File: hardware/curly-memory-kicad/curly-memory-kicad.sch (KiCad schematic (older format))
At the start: 18 parts

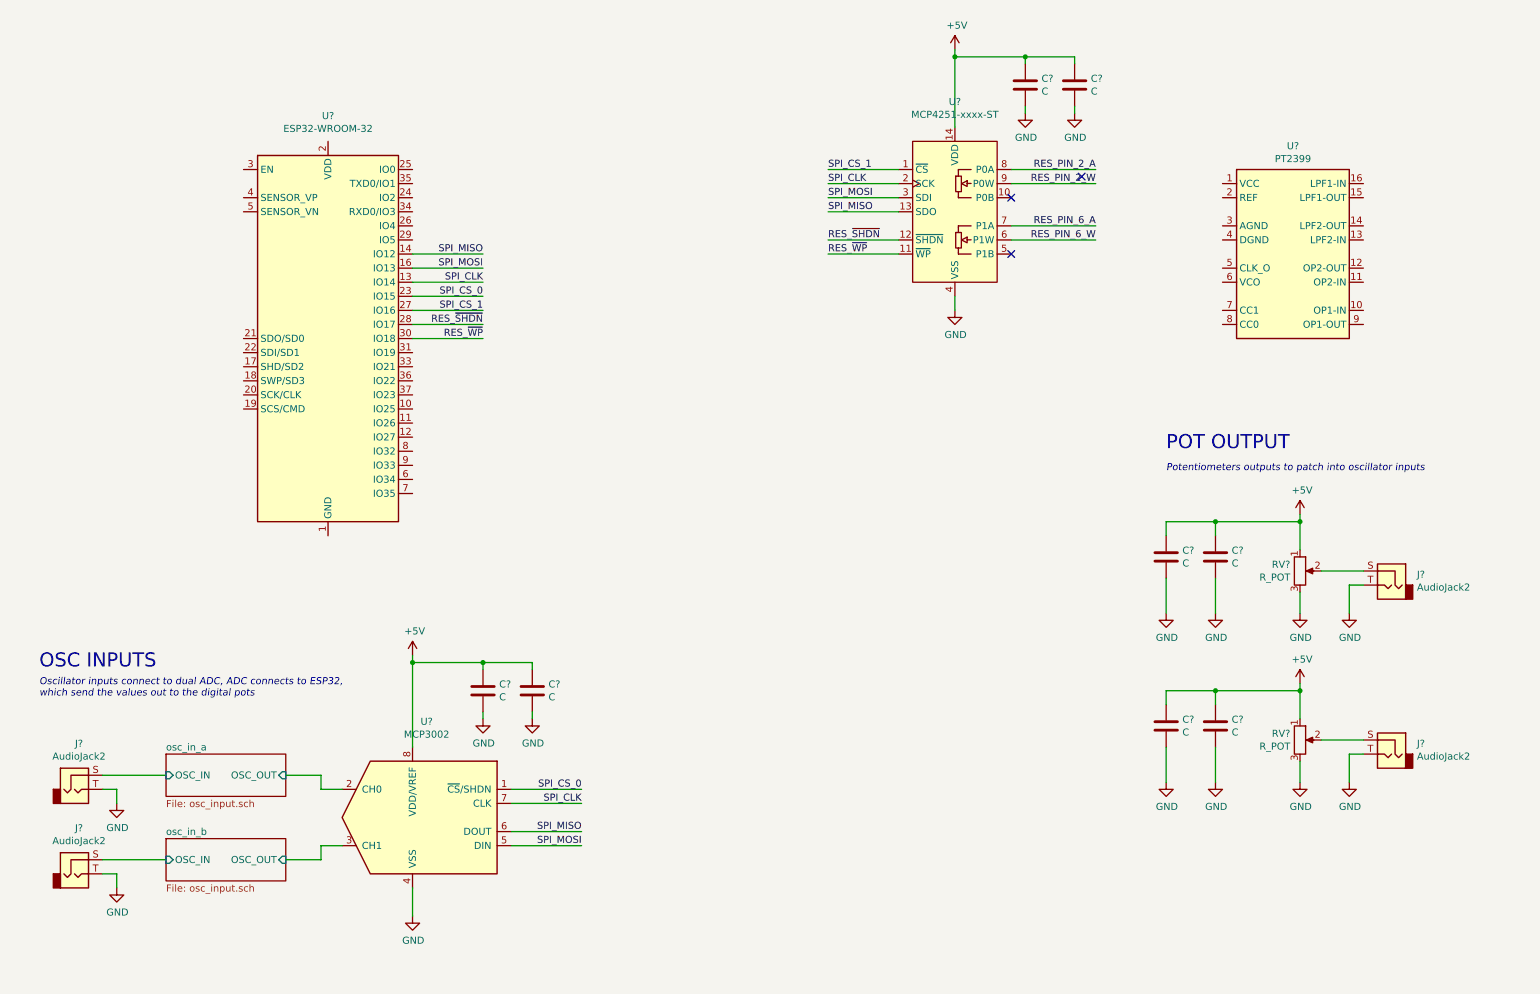
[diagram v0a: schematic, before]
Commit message: hardware update to relfect latest version of projectm gitignore updated to ignore *-bak files
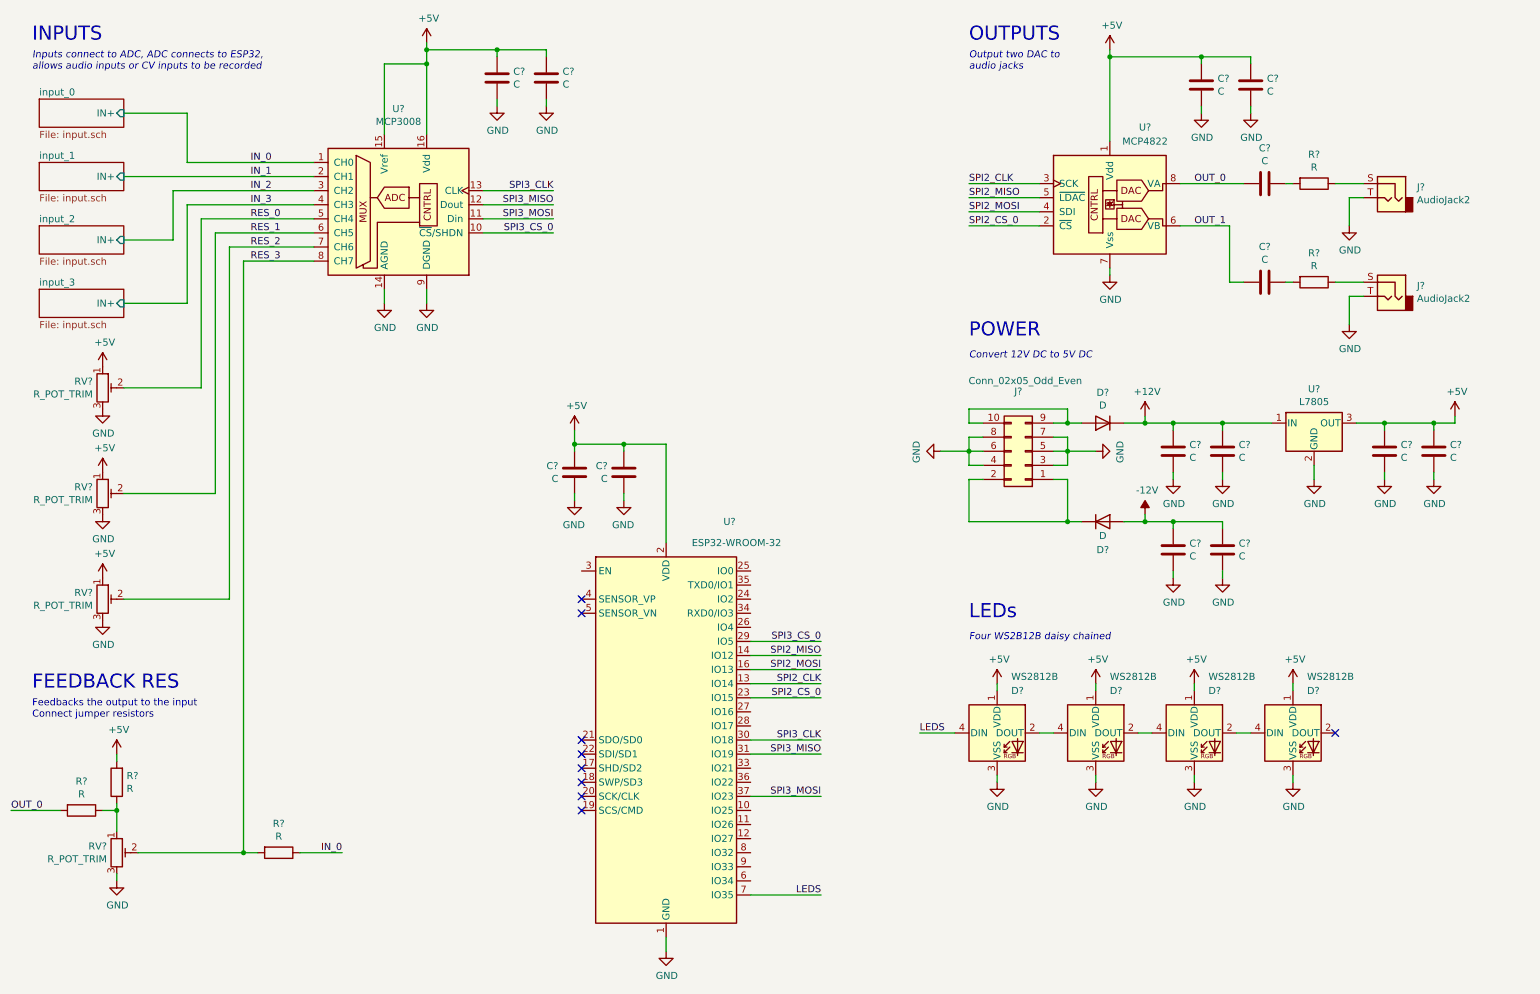
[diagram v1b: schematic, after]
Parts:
- removed C? (x6): C, symbol Device:C
- removed J? (x2): AudioJack2, symbol Connector:AudioJack2
- removed RV? (x2): R_POT, symbol Device:R_POT
- removed U?: MCP3002, symbol Analog_ADC:MCP3002
- removed U?: MCP4251-xxxx-ST, Package_SO:TSSOP-14_4.4x5mm_P0.65mm, symbol Potentiometer_Digital:MCP4251-xxxx-ST
- removed U?: PT2399, symbol Audio:PT2399
- added C? (x12): C, symbol Device:C
- added D? (x4): WS2812B, LED_SMD:LED_WS2812B_PLCC4_5.0x5.0mm_P3.2mm, symbol LED:WS2812B
- added D? (x2): D, symbol Device:D
- added J?: Conn_02x05_Odd_Even, symbol Connector_Generic:Conn_02x05_Odd_Even
- added R? (x5): R, symbol Device:R
- added RV? (x4): R_POT_TRIM, symbol Device:R_POT_TRIM
- added U?: MCP3008, symbol Analog_ADC:MCP3008
- added U?: MCP4822, symbol Analog_DAC:MCP4822
- added U?: L7805, symbol Regulator_Linear:L7805
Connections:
- net +5V: now also U?.2 (VDD), C?.1, C?.1, C?.1, C?.1, C?.1, C?.1, D?.1 (VDD), D?.1 (VDD), D?.1 (VDD), D?.1 (VDD), R?.2, RV?.1, RV?.1, RV?.1, U?.1 (Vdd), U?.15 (Vref), U?.16 (Vdd), U?.3 (OUT)
- net GND: now also U?.1 (GND), U?.15 (GND), U?.38 (GND), U?.39 (GND), C?.2, C?.2, C?.2, C?.2, C?.2, C?.2, C?.2, C?.2, C?.2, C?.2, D?.3 (VSS), D?.3 (VSS), D?.3 (VSS), D?.3 (VSS), J?.3 (Pin_3), J?.4 (Pin_4), J?.5 (Pin_5), J?.6 (Pin_6), J?.7 (Pin_7), J?.8 (Pin_8), RV?.3, RV?.3, RV?.3, RV?.3, U?.14 (AGND), U?.2 (GND), U?.7 (Vss), U?.9 (DGND)
- net SPI3_CS_0: now reaches U?.29 (IO5)
- net SPI3_CS_0: now also U?.10 (~CS~/SHDN)
- net SPI3_MISO: now reaches U?.31 (IO19)
- net SPI3_MISO: now also U?.12 (Dout)
- net SPI3_MOSI: now reaches U?.37 (IO23)
- net SPI3_MOSI: now also U?.11 (Din)
- net LEDS: now reaches U?.7 (IO35)
- net LEDS: now also D?.4 (DIN)
- net at J?.S: now also R?.1 (x2)
- net RES_~SHDN: no longer names the net of U?.28 (IO17)
- net RES_~WP renamed SPI3_CLK
- net SPI3_CLK: now also U?.13 (CLK)
- net SPI_CLK renamed SPI2_CLK
- net SPI2_CLK: now also U?.3 (SCK)
- net SPI_CS_0 renamed SPI2_CS_0
- net SPI2_CS_0: now also U?.2 (~CS)
- net SPI_CS_1: no longer names the net of U?.27 (IO16)
- net SPI_MISO renamed SPI2_MISO
- net SPI2_MISO: now also U?.5 (~LDAC)
- net SPI_MOSI renamed SPI2_MOSI
- net SPI2_MOSI: now also U?.4 (SDI)
- new net: R?.1, R?.1, RV?.1
- new net: D?.2 (DOUT), D?.4 (DIN) (x3)
- new net: C?.1, R?.2 (x2)
- new net: D?.1 (K), J?.1 (Pin_1), J?.2 (Pin_2)
- new net: D?.2 (A), J?.10 (Pin_10), J?.9 (Pin_9)
- new net +12V: C?.1, C?.1, D?.1 (K), U?.1 (IN)
- new net -12V: C?.1, C?.1, D?.2 (A)
- new net IN_0: R?.1, U?.1 (CH0)
- new net IN_1: U?.2 (CH1)
- new net IN_2: U?.3 (CH2)
- new net IN_3: U?.4 (CH3)
- new net OUT_0: C?.2, R?.2, U?.8 (VA)
- new net OUT_1: C?.2, U?.6 (VB)
- new net RES_0: RV?.2, U?.5 (CH4)
- new net RES_1: RV?.2, U?.6 (CH5)
- new net RES_2: RV?.2, U?.7 (CH6)
- new net RES_3: R?.2, RV?.2, U?.8 (CH7)
- no-connect marks 3 -> 9
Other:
- note added: "Convert 12V DC to 5V DC"
- note added: "FEEDBACK RES"
- note added: "Feedbacks the output to the input\nConnect jumper resistors"
- note added: "Four WS2B12B daisy chained"
- note added: "INPUTS"
- note added: "Inputs connect to ADC, ADC connects to ESP32,\nallows audio inputs or CV inputs to be recorded"
- note added: "LEDs"
- note added: "OUTPUTS"
- note added: "Output two DAC to\naudio jacks"
- note added: "POWER"
- note removed: "OSC INPUTS"
- note removed: "Oscillator inputs connect to dual ADC, ADC connects to ESP32,\nwhich send the values out to the digital pots"
- note removed: "POT OUTPUT"
- note removed: "Potentiometers outputs to patch into oscillator inputs"
- moved on the sheet: C?, J?, U?
